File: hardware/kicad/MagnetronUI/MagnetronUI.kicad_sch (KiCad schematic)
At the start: 10 parts, among them J1 Conn_01x04, J2 Conn_02x13_Counter_Clockwise, SW1 SW_Push, SW2 SW_Push

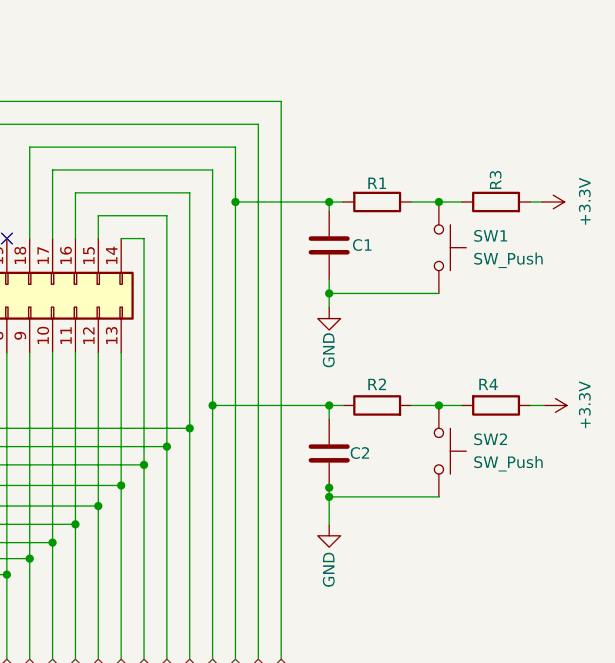
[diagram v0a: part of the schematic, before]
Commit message: feat: cleanup
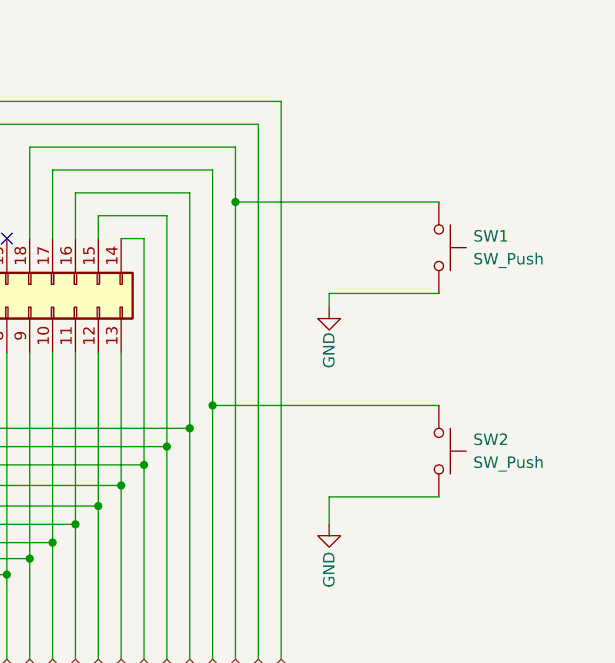
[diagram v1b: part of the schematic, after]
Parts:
- removed C1, C2: C, Capacitor_SMD:C_0805_2012Metric_Pad1.18x1.45mm_HandSolder, symbol Device:C
- removed R1, R2, R3, R4: R, Resistor_SMD:R_0805_2012Metric_Pad1.20x1.40mm_HandSolder, symbol Device:R
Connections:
- net aux1_btn: now also SW2.1
- net aux2_btn: now also SW1.1
